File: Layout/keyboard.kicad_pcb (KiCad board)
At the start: 2 copper layers, 340.5 x 86.5 mm, 180 parts, among them J1 Conn_01x04_Socket, J2 Conn_01x04_Socket, J3 Conn_01x04_Socket, J4 Conn_01x03_Socket, J5 Conn_01x03_Socket, J6 Conn_01x03_Socket, J7 Conn_01x04_Socket, J8 Conn_01x03_Socket

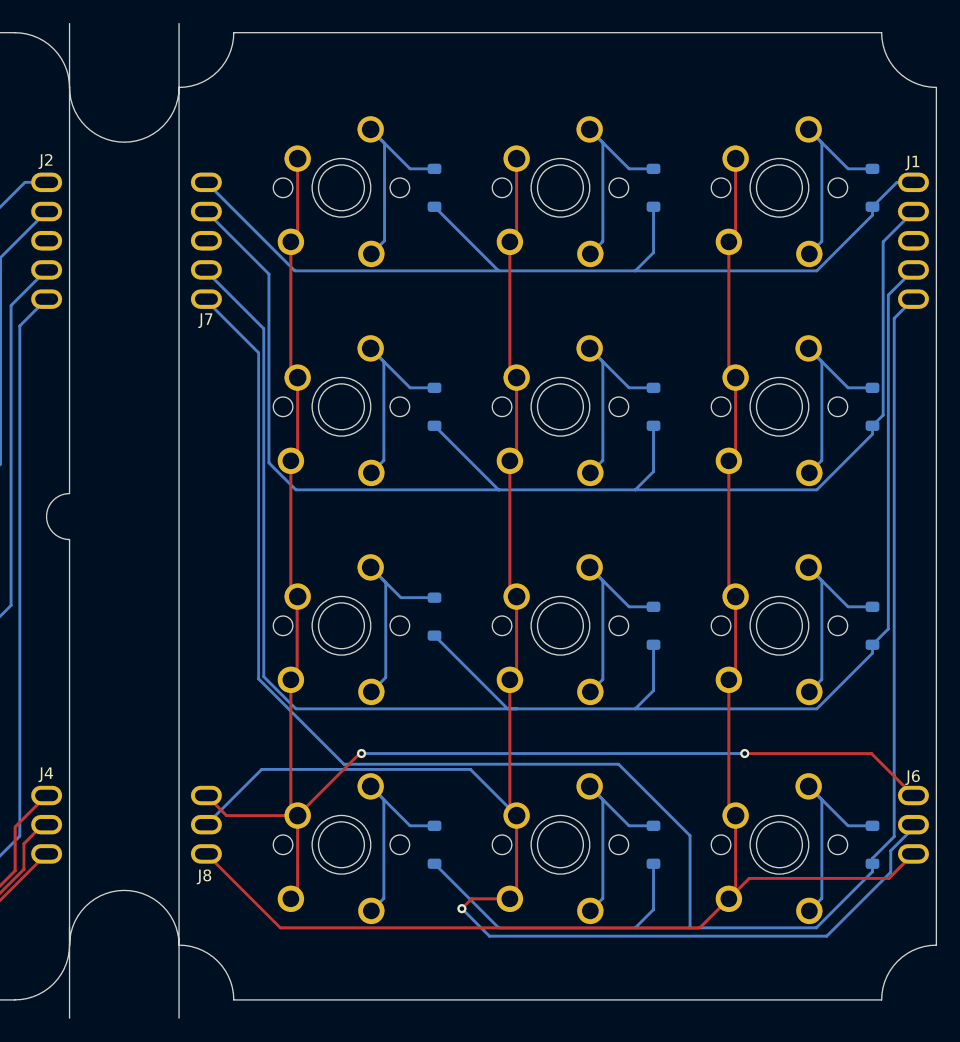
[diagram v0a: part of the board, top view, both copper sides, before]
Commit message: gerbers for seperate macropad and keyboard
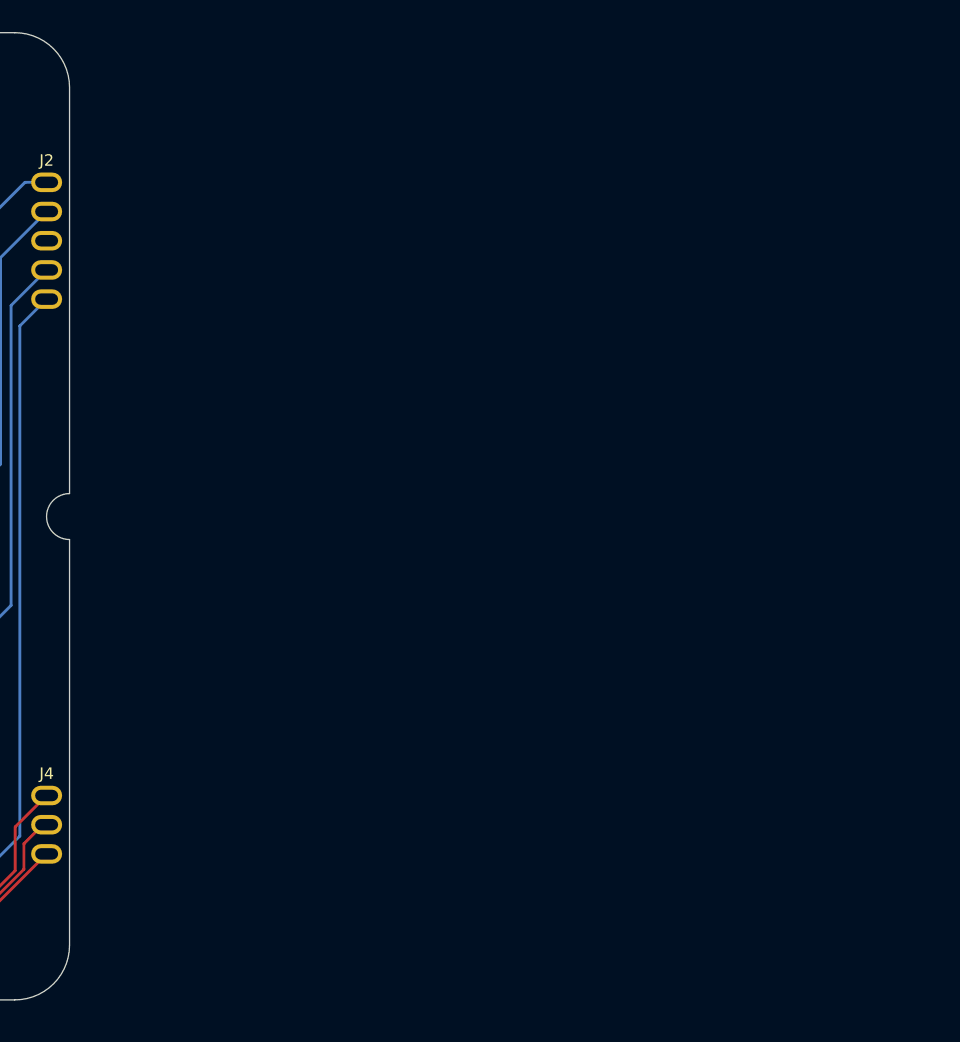
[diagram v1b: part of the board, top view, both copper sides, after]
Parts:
- removed D_10, D_11, D_12, D_13, D_2, D_3, D_4, D_5, D_6, D_7, D_8, D_9: D, Diode_SMD:D_SOD-123
- removed J1, J7: Conn_01x04_Socket, Connector_PinHeader_2.54mm:PinHeader_1x05_P2.54mm_Horizontal
- removed J6, J8: Conn_01x03_Socket, Connector_PinHeader_2.54mm:PinHeader_1x03_P2.54mm_Horizontal
- removed K_10, K_11, K_12, K_13, K_2, K_3, K_4, K_5, K_6, K_7, K_8, K_9: KEYSW, MX_Solderable:MX-Solderable-1U
- removed K_58, K_59, K_60, K_62, K_63, K_64, K_65, K_66, K_67, K_68: KEYSW, Gateron_KS33_Solderable:Gateron-KS33-Solderable-1U
- removed K_61, K_69: KEYSW, Gateron_KS33_Solderable:Gateron-KS33-Solderable-1.25U
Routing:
- net row3: track 606.8 -> 420.7 mm
- net col14: track 466.2 -> 319.3 mm, vias 2 -> 1
- net row2: track 616.5 -> 472.1 mm
- net col15: track 454.1 -> 321.2 mm
- net col13: track 448.8 -> 316.7 mm, vias 3 -> 1
- net row1: track 567.4 -> 452.8 mm
- net row0: track 516.3 -> 433.9 mm
- net Net-(D_2-A): track 18.8 -> 0.00 mm
- net Net-(D_9-A): track 18.7 -> 0.00 mm
- net Net-(D_7-A): track 18.7 -> 0.00 mm
- net Net-(D_5-A): track 18.7 -> 0.00 mm
- net Net-(D_3-A): track 18.7 -> 0.00 mm
- net Net-(D_6-A): track 18.7 -> 0.00 mm
- net Net-(D_8-A): track 18.7 -> 0.00 mm
- net Net-(D_13-A): track 18.7 -> 0.00 mm
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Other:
- board size 340.5 x 86.5 mm -> 265.1 x 84.1 mm
- board text removed: "V CUTS"
